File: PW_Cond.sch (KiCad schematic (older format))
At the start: 19 parts, among them J1 Conn_01x02_Female, J2 Conn_01x04_Female, J3 Conn_01x02_Female, U1 Opamp_Dual_Generic, U2 Opamp_Dual_Generic

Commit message: correct ampli op + tied up
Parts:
- removed D?: D_Zener, symbol device:D_Zener
- removed Q?: Q_NPN_BCE, symbol device:Q_NPN_BCE
- removed U1 (x2), U2, U?: Opamp_Dual_Generic, symbol device:Opamp_Dual_Generic
- added C? (x2): 100n, symbol Device:C
- added D?: 5.1V, symbol Device:D_Zener
- added Q?: BC847, Package_TO_SOT_SMD:SOT-23, symbol Transistor_BJT:BC847
- added U1, U2: MCP602, symbol Amplifier_Operational:MCP602
- R? (x9): symbol device:R -> PW_Cond-rescue:R-device
- R?: value R -> 5.1k; symbol device:R -> PW_Cond-rescue:R-device
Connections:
- wire segments 59 -> 79
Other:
- note added: "Alimentation et découplage"
- note added: "Amplificateur d’instrumentation"
- note added: "Source de courant 1mA"
- moved on the sheet: J1, J2, J3

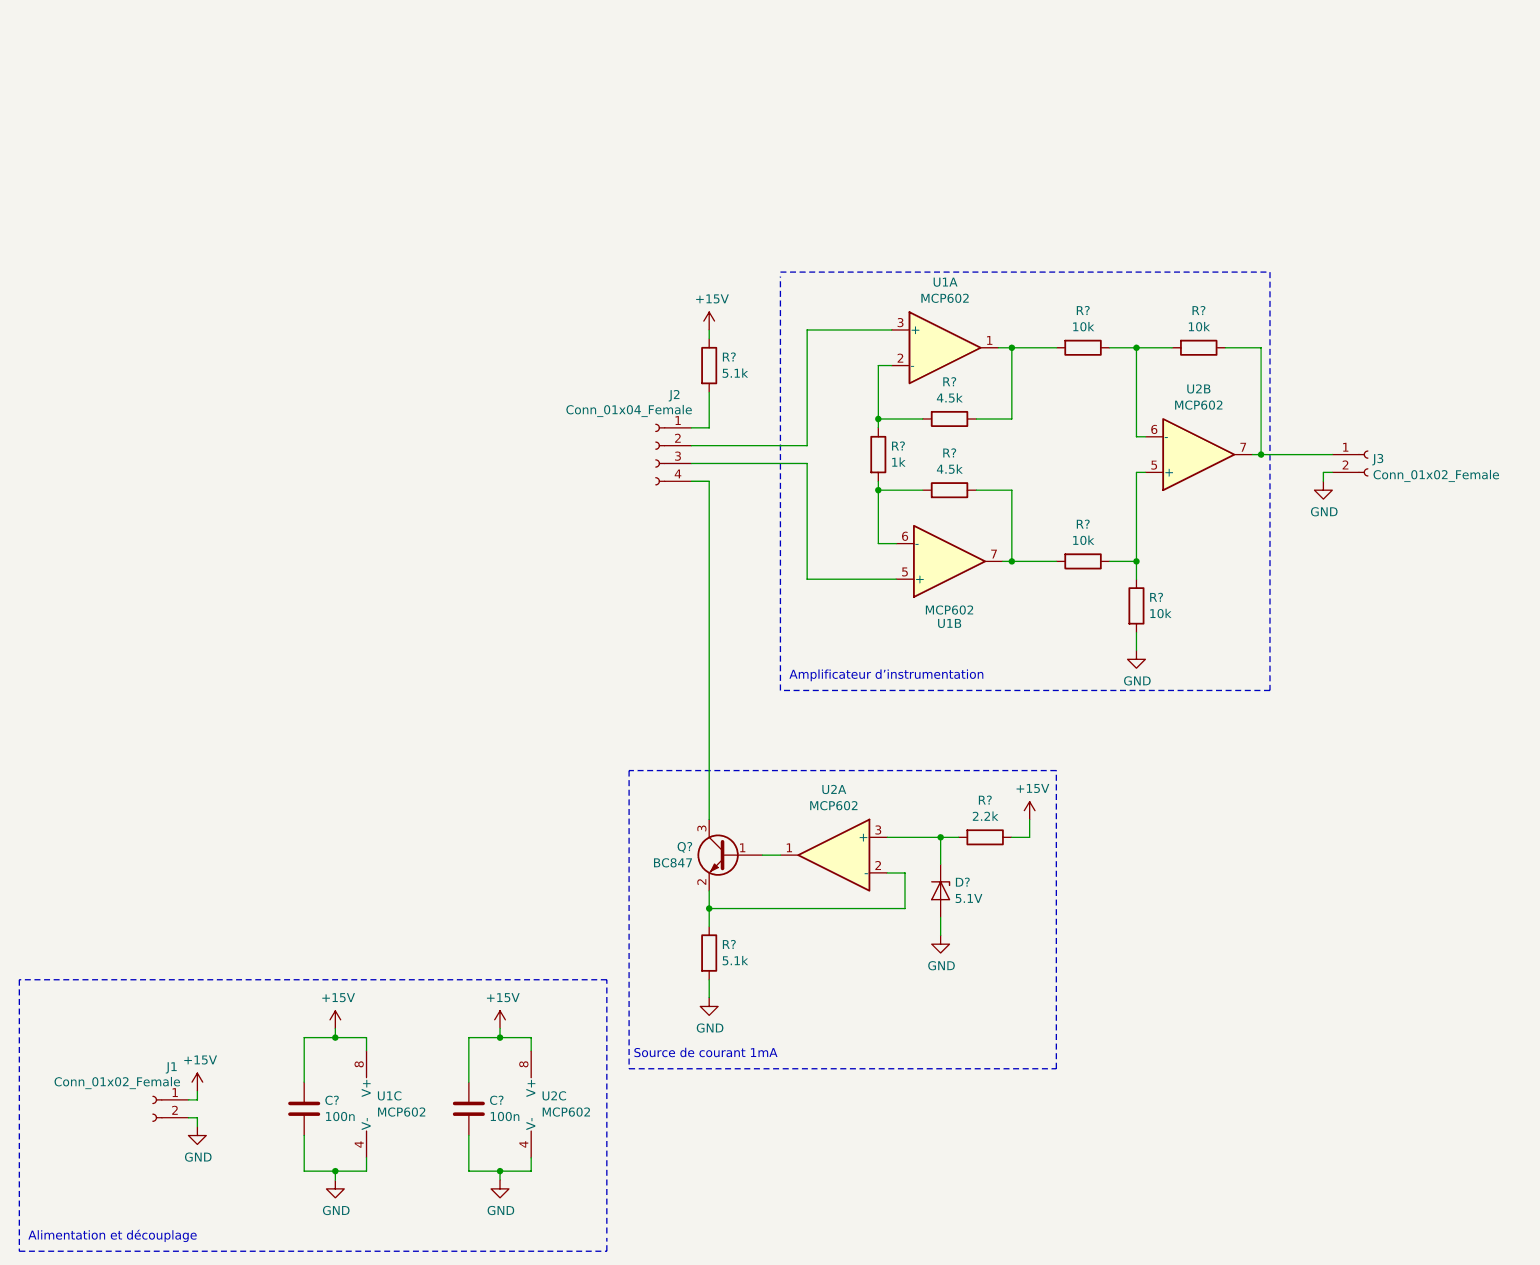
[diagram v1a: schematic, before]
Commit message: added footprints and an LED git add *
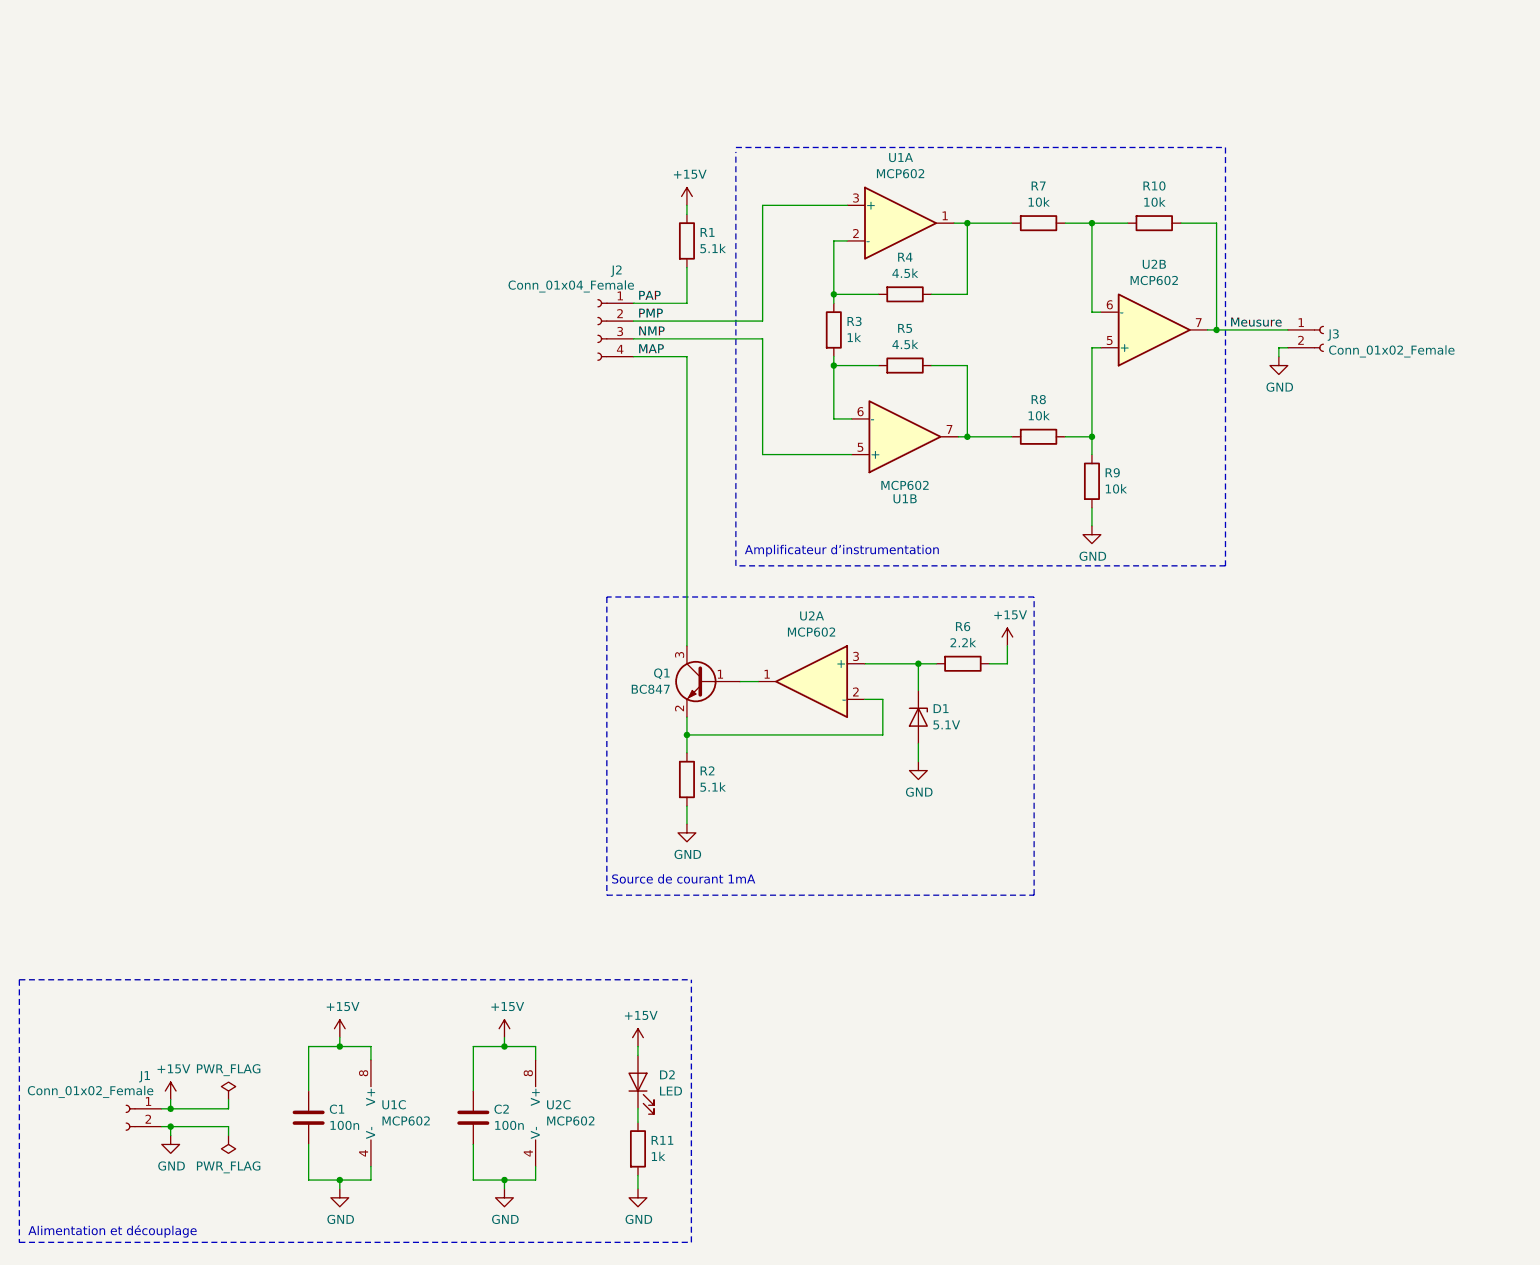
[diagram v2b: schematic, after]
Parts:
- added D2: LED, LED_THT:LED_D3.0mm, symbol Device:LED
- added R11: 1k, Resistor_SMD:R_0805_2012Metric_Pad1.15x1.40mm_HandSolder, symbol Device:R
- C1, C2: renamed from C?; footprint (none) -> Capacitor_SMD:C_0805_2012Metric_Pad1.15x1.40mm_HandSolder
- D1: renamed from D?; footprint (none) -> Diode_SMD:D_SOD-123
- J1, J3: footprint (none) -> Connector_PinHeader_2.54mm:PinHeader_1x02_P2.54mm_Vertical
- J2: footprint (none) -> Connector_PinHeader_2.54mm:PinHeader_1x04_P2.54mm_Vertical
- R1, R10, R2, R3, R4, R5, R6, R7, R8, R9: renamed from R?; footprint (none) -> Resistor_SMD:R_0805_2012Metric_Pad1.15x1.40mm_HandSolder
- U1, U2: footprint (none) -> Package_SO:SOIC-8_3.9x4.9mm_P1.27mm
- gave numbers to parts that had none: 1
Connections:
- net +15V: now also D2.2 (A)
- net GND: now also R11.2
- net PMP: now reaches J2.2 (Pin_2), U1.3 (+)
- net Meusure: now reaches J3.1 (Pin_1), R10.1, U2.7
- net PAP: now reaches J2.1 (Pin_1), R1.2
- net NMP: now reaches J2.3 (Pin_3), U1.5 (+)
- net MAP: now reaches J2.4 (Pin_4), Q1.3 (C)
- new net: D2.1 (K), R11.1
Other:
- moved on the sheet: C1, C2, D1, J1, J2, J3, Q1, R1, R10, R2, R3, R4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

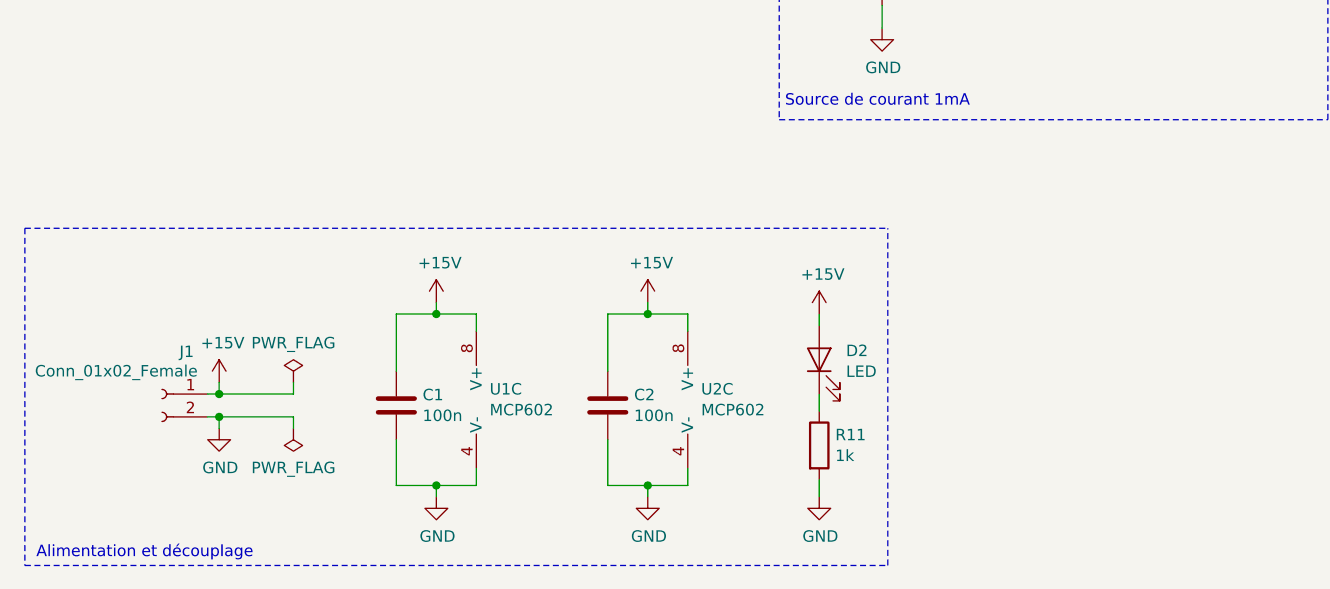
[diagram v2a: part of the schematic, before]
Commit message: minor cleanup + started pcb
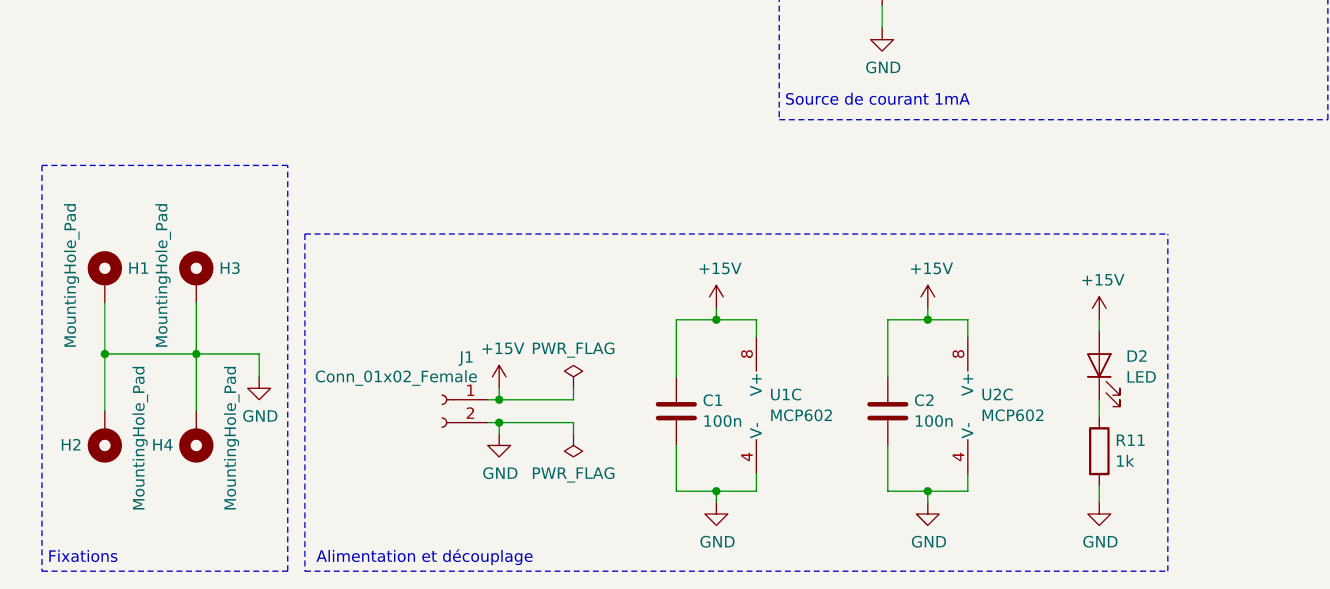
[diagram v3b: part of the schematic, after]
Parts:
- added H1, H2, H3, H4: MountingHole_Pad, MountingHole:MountingHole_3.2mm_M3_Pad_Via, symbol Mechanical:MountingHole_Pad
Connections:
- net GND: now also H1.1, H2.1, H3.1, H4.1
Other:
- note added: "Fixations"
- moved on the sheet: C1, C2, D2, J1, R11, U1C, U2C

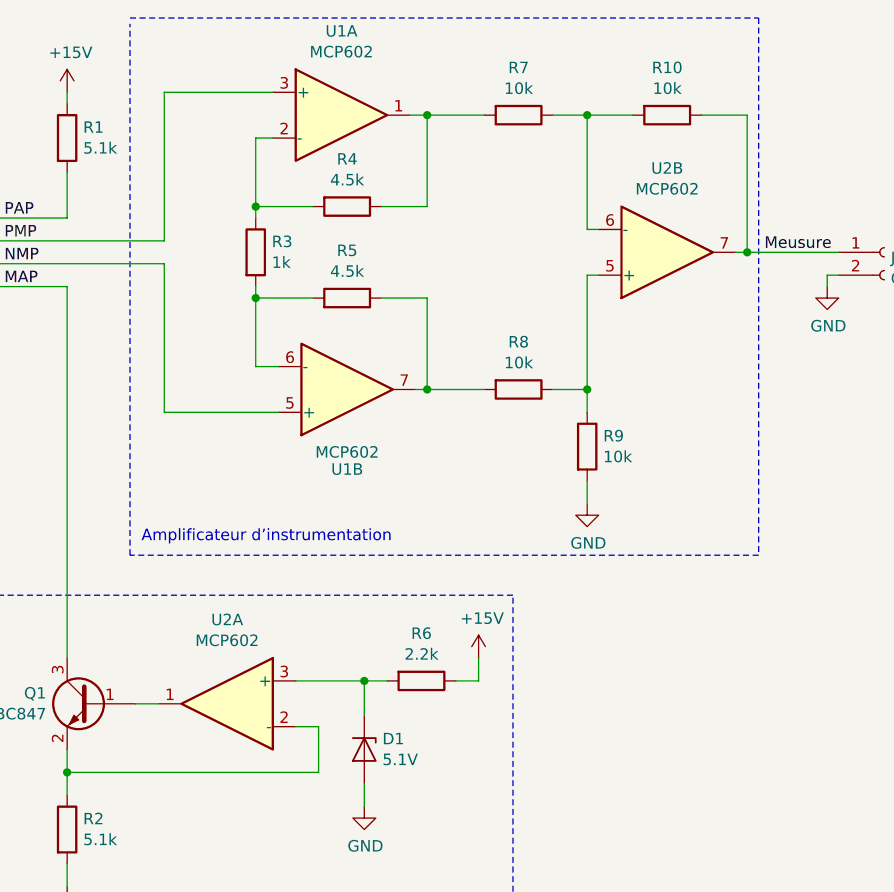
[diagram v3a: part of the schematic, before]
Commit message: psb is going well
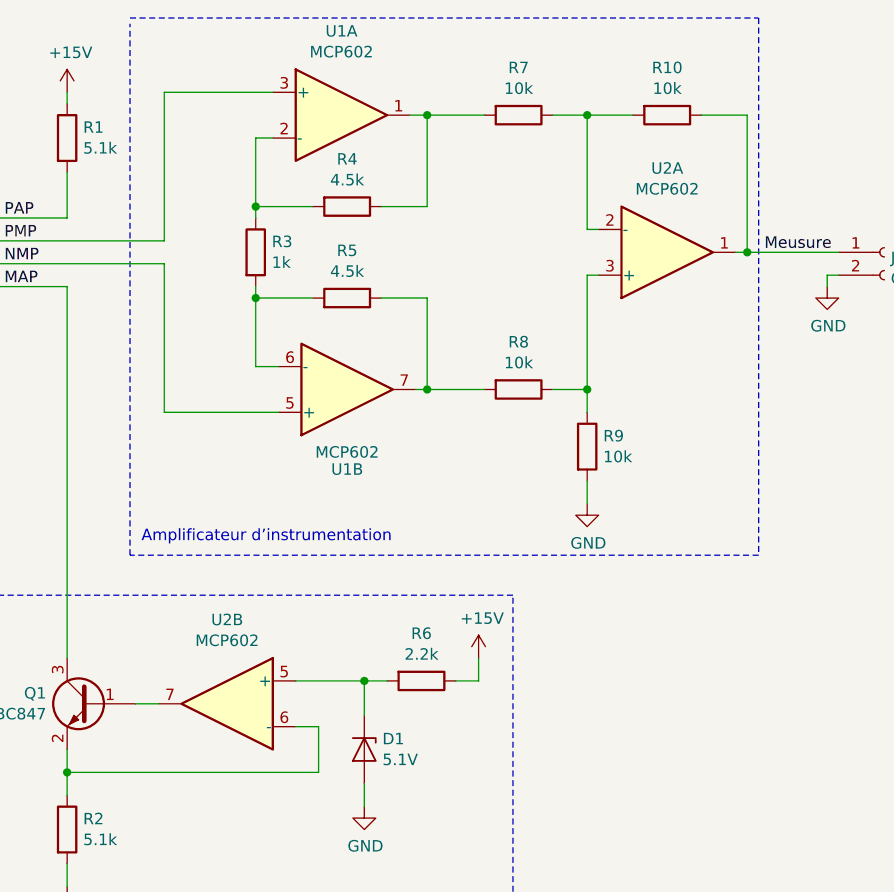
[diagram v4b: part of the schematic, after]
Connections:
- net Meusure: now also U2.1; no longer U2.7
- net at R10.2, R7.1: now also U2.2 (-); no longer U2.6 (-)
- net at R8.1, R9.1: now also U2.3 (+); no longer U2.5 (+)
- net at Q1.2 (E), R2.1: now also U2.6 (-); no longer U2.2 (-)
- net at Q1.1 (B): now also U2.7; no longer U2.1
- net at D1.1 (K), R6.2: now also U2.5 (+); no longer U2.3 (+)
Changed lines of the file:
@@
 $Comp
 L Amplifier_Operational:MCP602 U2
-U 2 1 61044EEE
+U 1 1 61044EEE
 P 6875 2550
 F 0 "U2" H 6875 2183 50  0000 C CNN
@@
 F 2 "Package_SO:SOIC-8_3.9x4.9mm_P1.27mm" H 6875 2550 50  0001 C CNN
 F 3 "http://ww1.microchip.com/downloads/en/DeviceDoc/21314g.pdf" H 6875 2550 50  0001 C CNN
-	2    6875 2550
+	1    6875 2550
 	1    0    0    1
 $EndComp
 $Comp
 L Amplifier_Operational:MCP602 U2
-U 1 1 61049572
+U 2 1 61049572
 P 4950 4525
 F 0 "U2" H 4950 4892 50  0000 C CNN
@@
 F 2 "Package_SO:SOIC-8_3.9x4.9mm_P1.27mm" H 4950 4525 50  0001 C CNN
 F 3 "http://ww1.microchip.com/downloads/en/DeviceDoc/21314g.pdf" H 4950 4525 50  0001 C CNN
-	1    4950 4525
+	2    4950 4525
 	-1   0    0    -1
 $EndComp
